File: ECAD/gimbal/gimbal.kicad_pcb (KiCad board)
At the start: 2 copper layers, 47.6 x 39.4 mm, 15 parts, among them J1 PWR, J2 UPDI, J3 BNO1, J4 Servo, J5 UART, J6 NOTIF, J7 Servo, J8 BNO2, J9 Servo, U1 LM1117-3.3, U2 ATtiny1604-SS

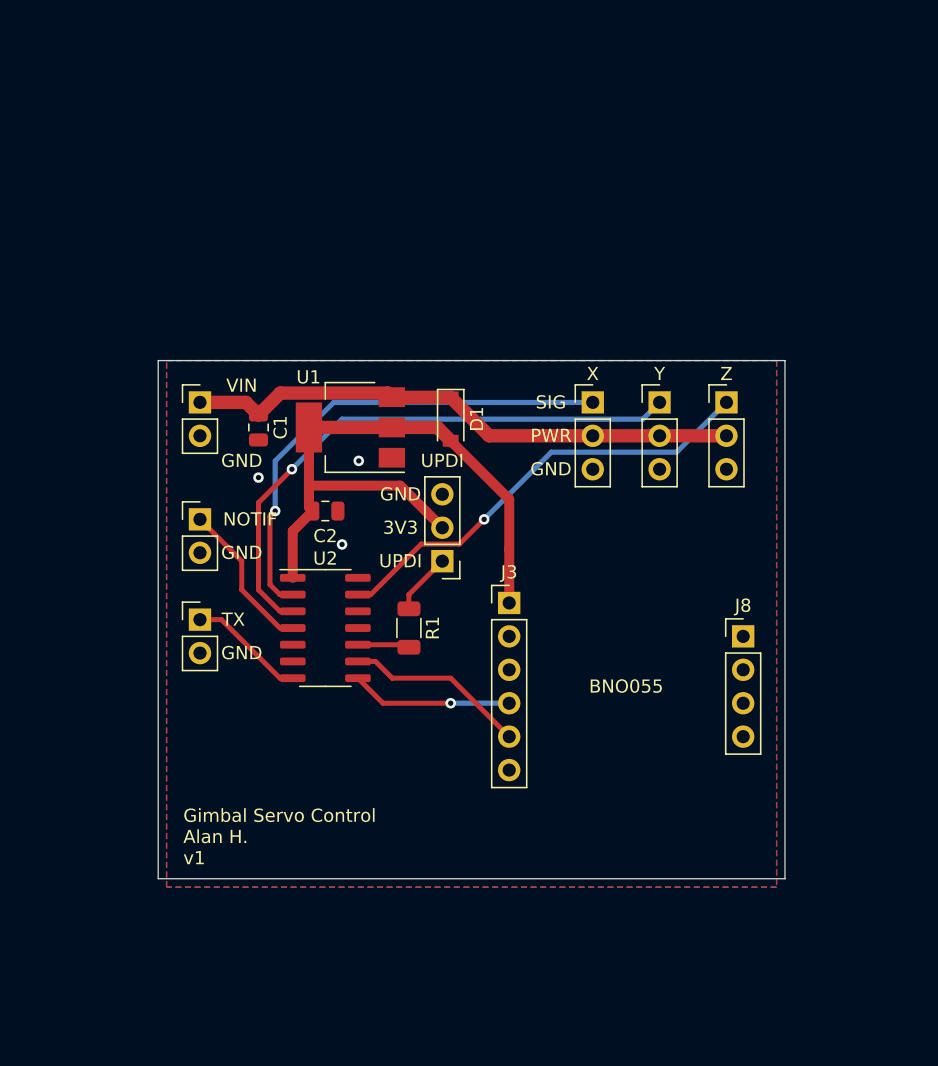
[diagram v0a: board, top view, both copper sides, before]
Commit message: v2 for A5100 gimbal
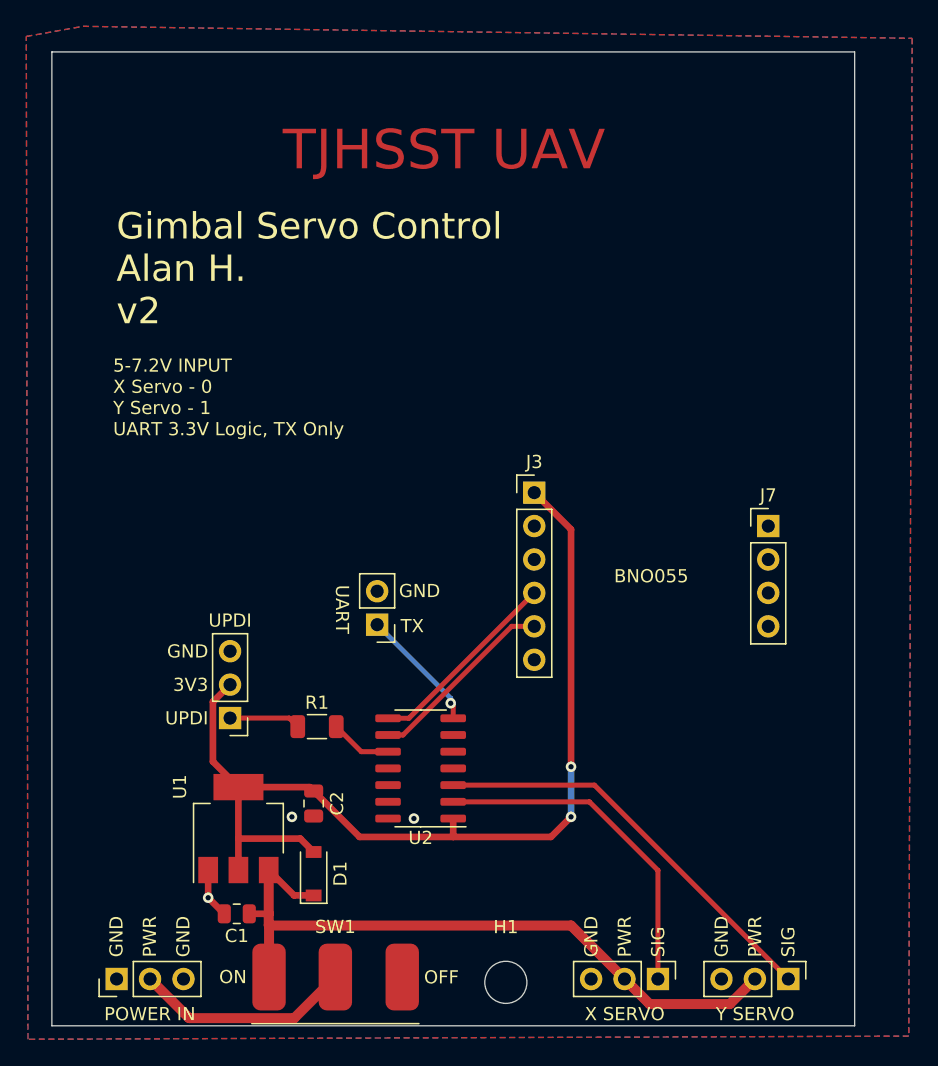
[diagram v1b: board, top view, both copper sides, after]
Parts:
- removed the J6 at (128.9, 87.0)
- removed J9: Servo, Connector_PinHeader_2.54mm:PinHeader_1x03_P2.54mm_Vertical
- added H1: MountingHole, MountingHole:MountingHole_3.2mm_M3, F.Cu at (152.1, 122.2)
- added SW1: POWER, gimbal:Switch, F.Cu at (139.2, 121.8)
- D1: value MBR0520LT1G -> BAT54
- J1: footprint Connector_PinHeader_2.54mm:PinHeader_1x02_P2.54mm_Vertical -> Connector_PinHeader_2.54mm:PinHeader_1x03_P2.54mm_Vertical
- moved J6 44.9 mm to (173.6, 121.9), turned to -90 degrees
- moved J1 44.3 mm to (122.6, 121.9), turned to 90 degrees
- moved J4 44.1 mm to (163.7, 121.9), turned to -90 degrees
- moved C1 37.0 mm to (131.7, 117.0), turned to 180 degrees
- moved D1 36.1 mm to (137.5, 113.9), turned to 90 degrees
- moved U1 31.6 mm to (131.8, 110.5), turned to 90 degrees
- moved C2 22.2 mm to (137.5, 108.6), turned to -90 degrees
- moved J2 20.1 mm to (131.2, 102.1)
- moved J5 13.5 mm to (142.4, 95.0), turned to 180 degrees
- moved U2 12.9 mm to (145.7, 105.9), turned to 180 degrees
- moved R1 10.2 mm to (137.8, 102.7), turned to 0 degrees
- moved J3 8.60 mm to (154.3, 85.0)
- moved J7 8.60 mm to (172.1, 87.5)
- renumbered J7 to J6, J8 to J7
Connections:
- J1 pad 1: VCC -> GND
- J1 pad 2: GND -> Net-(J1-Pad2)
- J3 pad 2: (no net) -> unconnected-(J3-Pad2)
- J3 pad 6: (no net) -> unconnected-(J3-Pad6)
- J7 pad 1: (no net) -> unconnected-(J7-Pad1)
- J7 pad 2: (no net) -> unconnected-(J7-Pad2)
- J7 pad 3: (no net) -> unconnected-(J7-Pad3)
- J7 pad 4: (no net) -> unconnected-(J7-Pad4)
- U2 pad 11: (no net) -> unconnected-(U2-Pad11)
- U2 pad 12: (no net) -> unconnected-(U2-Pad12)
- U2 pad 13: /Servo_Z -> unconnected-(U2-Pad13)
- U2 pad 4: /NOTIF -> unconnected-(U2-Pad4)
- U2 pad 5: (no net) -> unconnected-(U2-Pad5)
- U2 pad 6: (no net) -> unconnected-(U2-Pad6)
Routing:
- net /Servo_Z: track 34.1 -> 0.00 mm, vias 1 -> 0
- net +3V3: track 49.0 -> 76.2 mm, vias 0 -> 2
- net Net-(J1-Pad2): track 0.00 -> 16.6 mm
- net /Servo_Y: track 43.5 -> 31.6 mm, vias 1 -> 0
- net /NOTIF: track 11.7 -> 0.00 mm
- net /Servo_X: track 37.6 -> 26.0 mm, vias 1 -> 0
- net VCC: track 42.4 -> 54.0 mm
- net GND: track 0.00 -> 3.83 mm
- net /SDA: track 12.3 -> 15.1 mm, vias 1 -> 0
- net Net-(R1-Pad2): track 3.95 -> 4.73 mm
- net /UPDI: track 4.67 -> 5.41 mm
- net /SCL: track 13.9 -> 14.5 mm
- net /TX: track 8.89 -> 9.50 mm, vias 0 -> 1
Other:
- board size 47.6 x 39.4 mm -> 61 x 74 mm
- net class Default removed
- board text added: "5-7.2V INPUT X Servo - 0 Y Servo - 1 UART 3.3V Logic, TX Only"
- board text added: "Gimbal Servo Control Alan H. v2"
- board text added: "POWER IN"
- board text added: "TJHSST UAV"
- board text added: "UART"
- board text added: "X SERVO"
- board text added: "Y SERVO"
- board text removed: "Gimbal Servo Control Alan H. v1"
- board text removed: "NOTIF"
- board text removed: "VIN"
- board text removed: "X"
- board text removed: "Y"
- board text removed: "Z"
